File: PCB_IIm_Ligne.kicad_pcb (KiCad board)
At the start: 2 copper layers, 100 x 100 mm, 37 parts, among them J1 Screw_Terminal_01x08, J2 Screw_Terminal_01x08, J3 Screw_Terminal_01x08, J4 Screw_Terminal_01x08, K1 G2RK-2 DC12, K2 Relay_DPDT_Latching_2coil, Q2 MPSA56, Q3 BC557B, Q4 BC557B, Q5 2N3904, Q6 IRF40B207, U2 TLC555xP

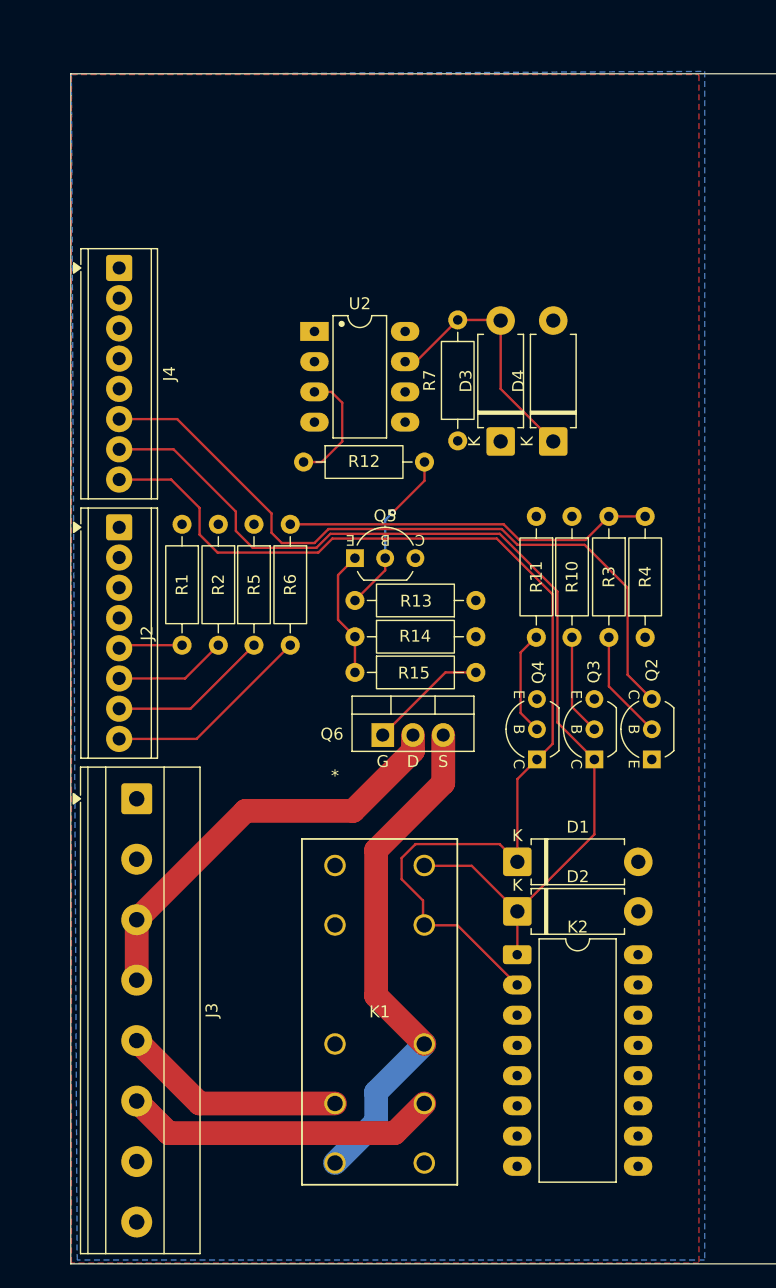
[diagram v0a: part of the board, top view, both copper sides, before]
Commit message: Schematic V1
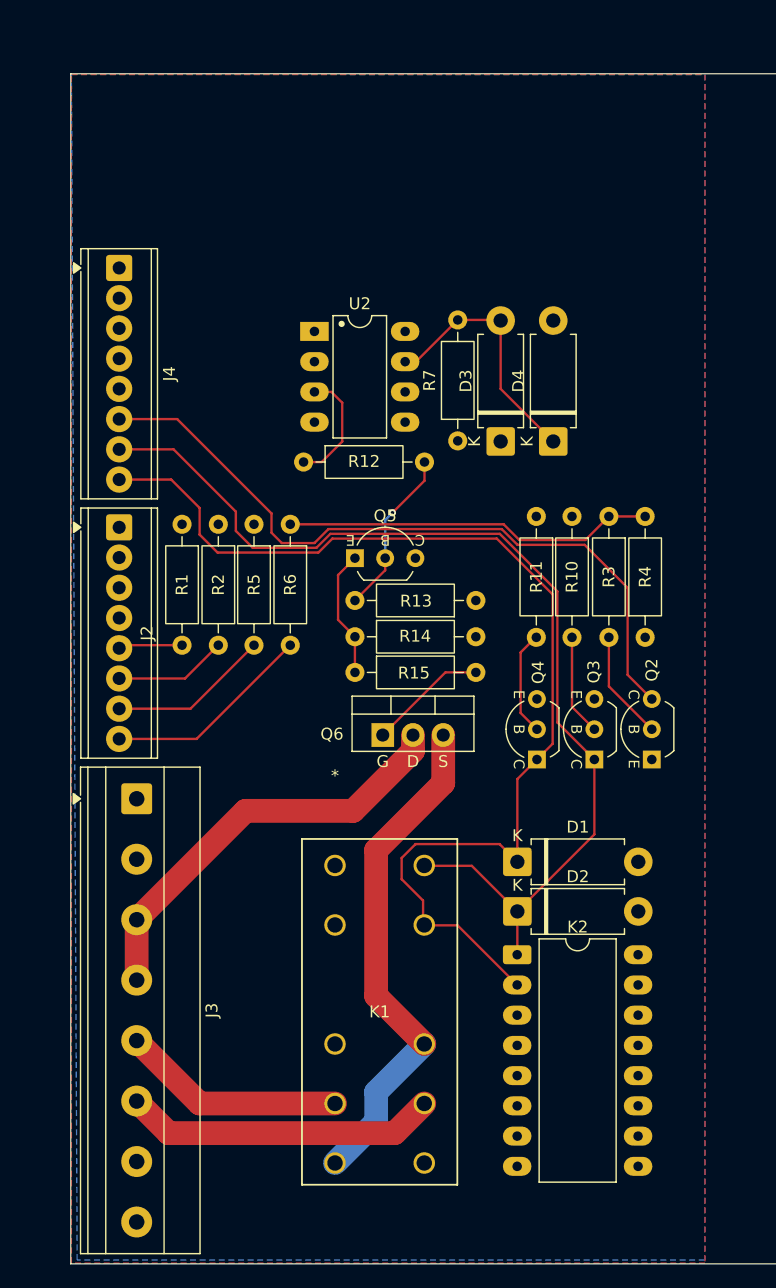
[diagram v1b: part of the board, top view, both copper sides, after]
